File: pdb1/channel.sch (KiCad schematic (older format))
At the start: 6 parts, among them P1 CONN_XT60, P2 CONN_XT60, P3 CONN_02X03, P6 CONN_XT60, P7 CONN_XT60, P8 CONN_XT60

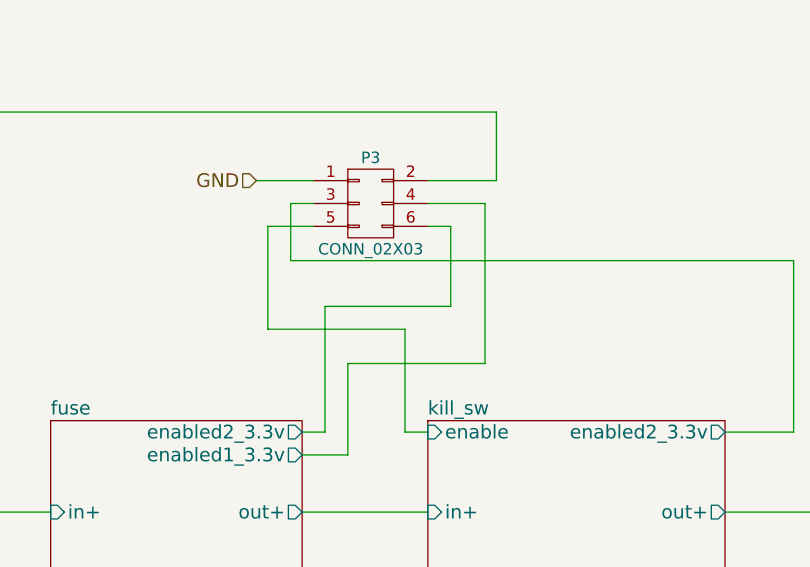
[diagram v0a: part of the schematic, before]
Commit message: test
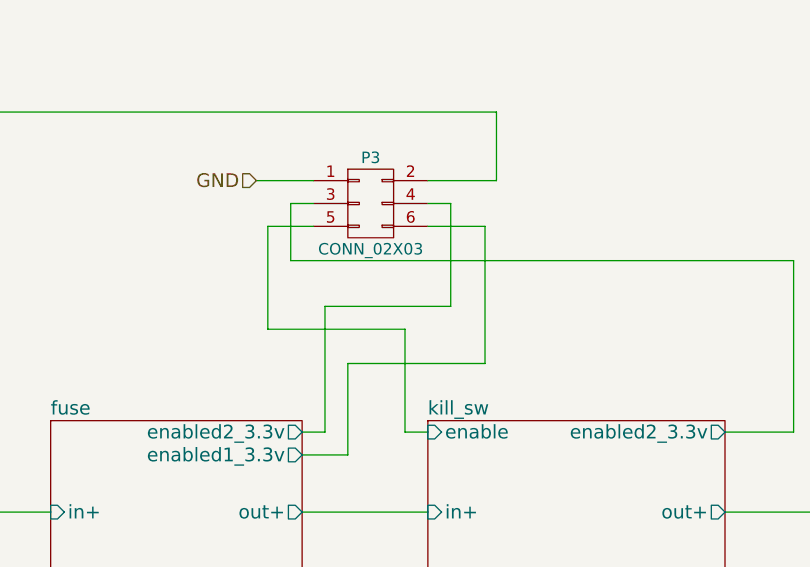
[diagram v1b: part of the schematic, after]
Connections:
- net fuse/enabled1_3.3v: now also P3.6 (P6); no longer P3.4 (P4)
- net fuse/enabled2_3.3v: now also P3.4 (P4); no longer P3.6 (P6)
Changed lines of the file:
@@
 	5950 3450 5950 3050
 Wire Wire Line
-	5850 2800 6400 2800
+	6400 2800 5850 2800
 Wire Wire Line
-	6400 2800 6400 2450
-Wire Wire Line
-	6400 2450 6300 2450
+	6400 2350 6400 2800
 Wire Wire Line
 	6200 2900 5600 2900
@@
 	5950 3050 6550 3050
 Wire Wire Line
-	6550 3050 6550 2350
-Wire Wire Line
-	6550 2350 6300 2350
+	6550 3050 6550 2450
 Wire Wire Line
 	7900 2600 5700 2600
@@
 Wire Wire Line
 	1950 1250 1650 1250
+Wire Wire Line
+	6400 2350 6300 2350
+Wire Wire Line
+	6550 2450 6300 2450
 $EndSCHEMATC
